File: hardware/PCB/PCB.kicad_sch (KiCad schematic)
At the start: 41 parts, among them J1 Conn_01x02_Pin, J2 USB_C_Receptacle_USB2.0_14P, Q1 BC807, Q2 BC817, Q3 BC817, SW1 SW_Push, SW2 SW_Push, U1 ESP32-C6-MINI-1, U2 AP3015, U3 MCP1700x-330xxTT

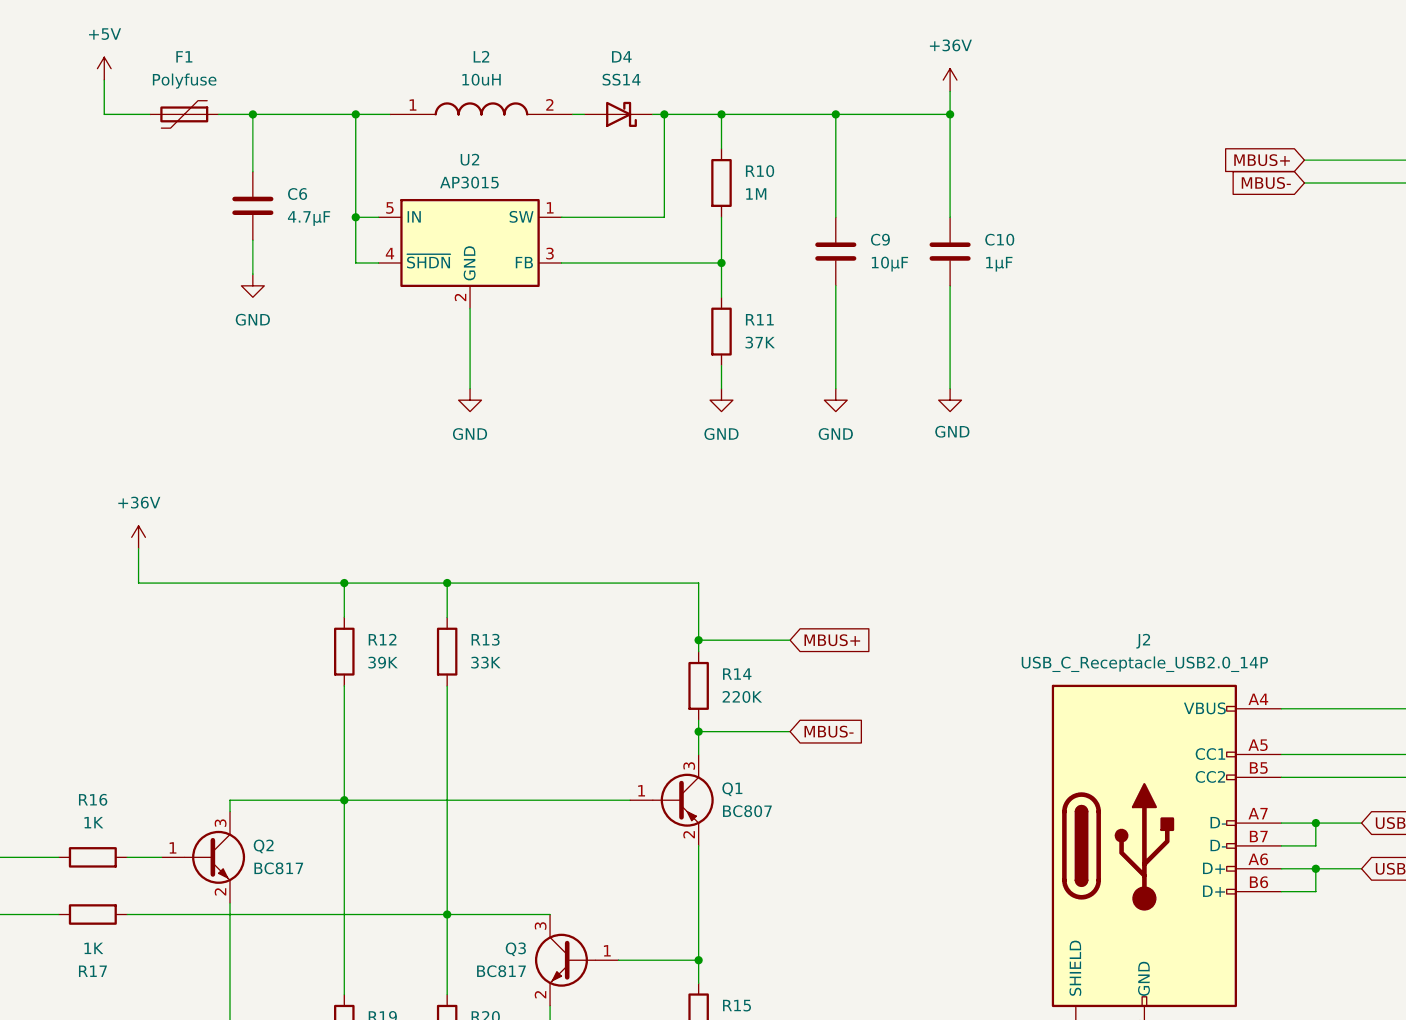
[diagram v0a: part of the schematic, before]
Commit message: WIP - Adding BOM
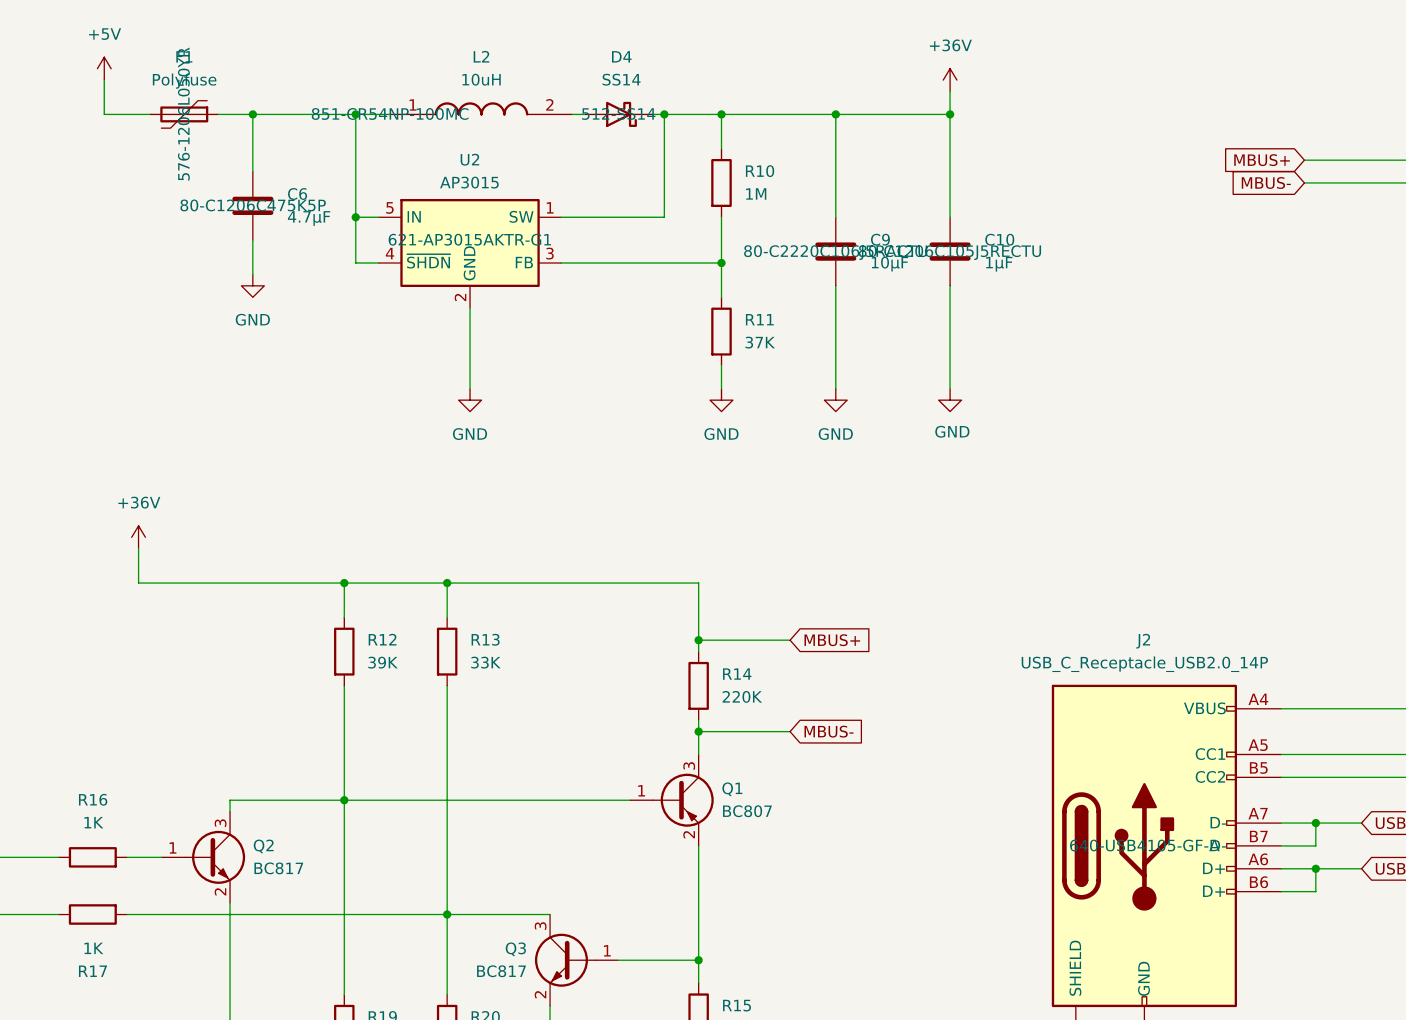
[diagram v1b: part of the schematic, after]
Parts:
- C1: Mouse_PN (none) -> 80-C0805C104J4RAUTO
- C10: footprint Capacitor_SMD:C_0805_2012Metric -> Capacitor_SMD:C_1206_3216Metric; Mouse_PN (none) -> 80-C1206C105J5RECTU
- C2: Mouse_PN (none) -> 80-C0805C226M8P7210
- C3, C5, C7: Mouse_PN (none) -> 80-C0805C105J4RACLR
- C6: footprint Capacitor_SMD:C_0805_2012Metric -> Capacitor_SMD:C_1206_3216Metric; Mouse_PN (none) -> 80-C1206C475K5P
- C9: footprint Capacitor_SMD:C_0805_2012Metric -> Capacitor_SMD:C_1206_3216Metric; Mouse_PN (none) -> 80-C2220C106J5RACTU
- D1, D2, D3: Mouse_PN (none) -> 630-HSMH-H170
- D4: Mouse_PN (none) -> 512-SS14
- F1: Mouse_PN (none) -> 576-1206L050YR
- J2: Mouse_PN (none) -> 640-USB4105-GF-A
- L2: Mouse_PN (none) -> 851-CR54NP-100MC
- R3, R4, R6, R7, R8: Mouse_PN (none) -> 667-ERA-6ARW512V
- SW1, SW2: Mouse_PN (none) -> 640-SWT0110020010SSA
- U1: Mouse_PN (none) -> 356-ESP32-C6MINI1UH4
- U2: Mouse_PN (none) -> 621-AP3015AKTR-G1
- U3: Mouse_PN (none) -> 579-MCP1700T3302E/TT
